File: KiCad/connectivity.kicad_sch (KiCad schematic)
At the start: 28 parts, among them IC17 GM02SP, U11 MAX98357A, U17 CXD5610GF, U18 ESP32-C6, U19 HP5354.A, U21 BGA524N6, U23 BGA524N6, Y1 WE-SPXO_CFPS-39, Y3 ECS-TXO-20CSMV4-260-AN-TR

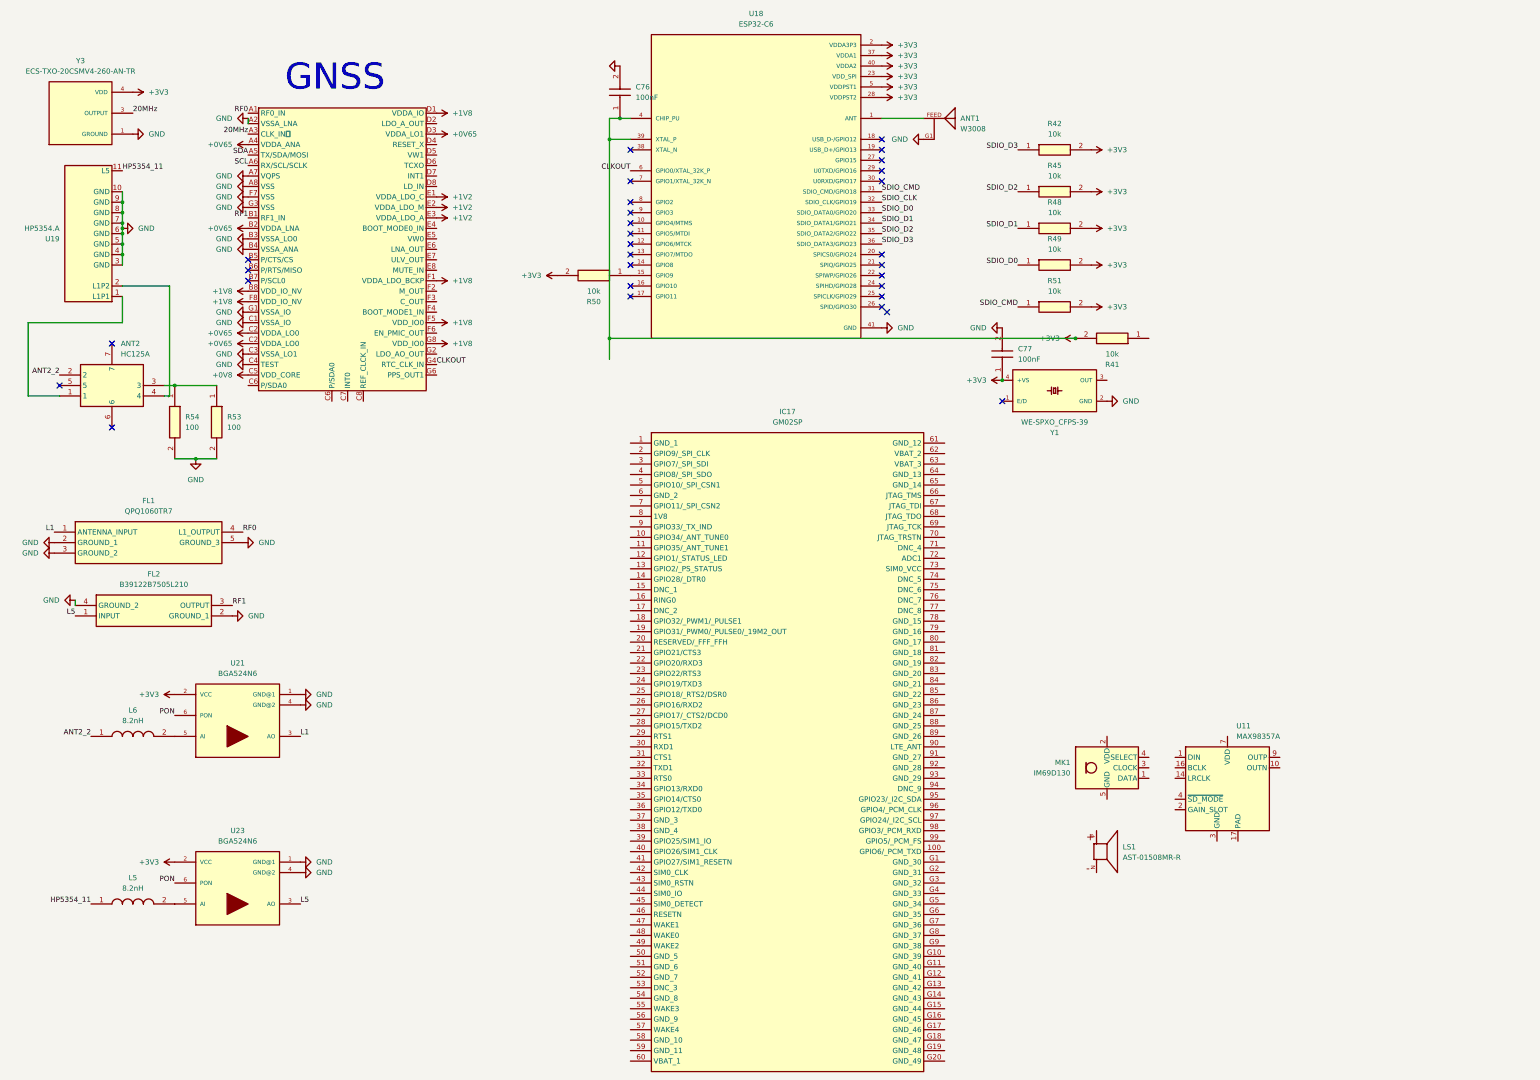
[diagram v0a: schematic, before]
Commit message: continue redesign
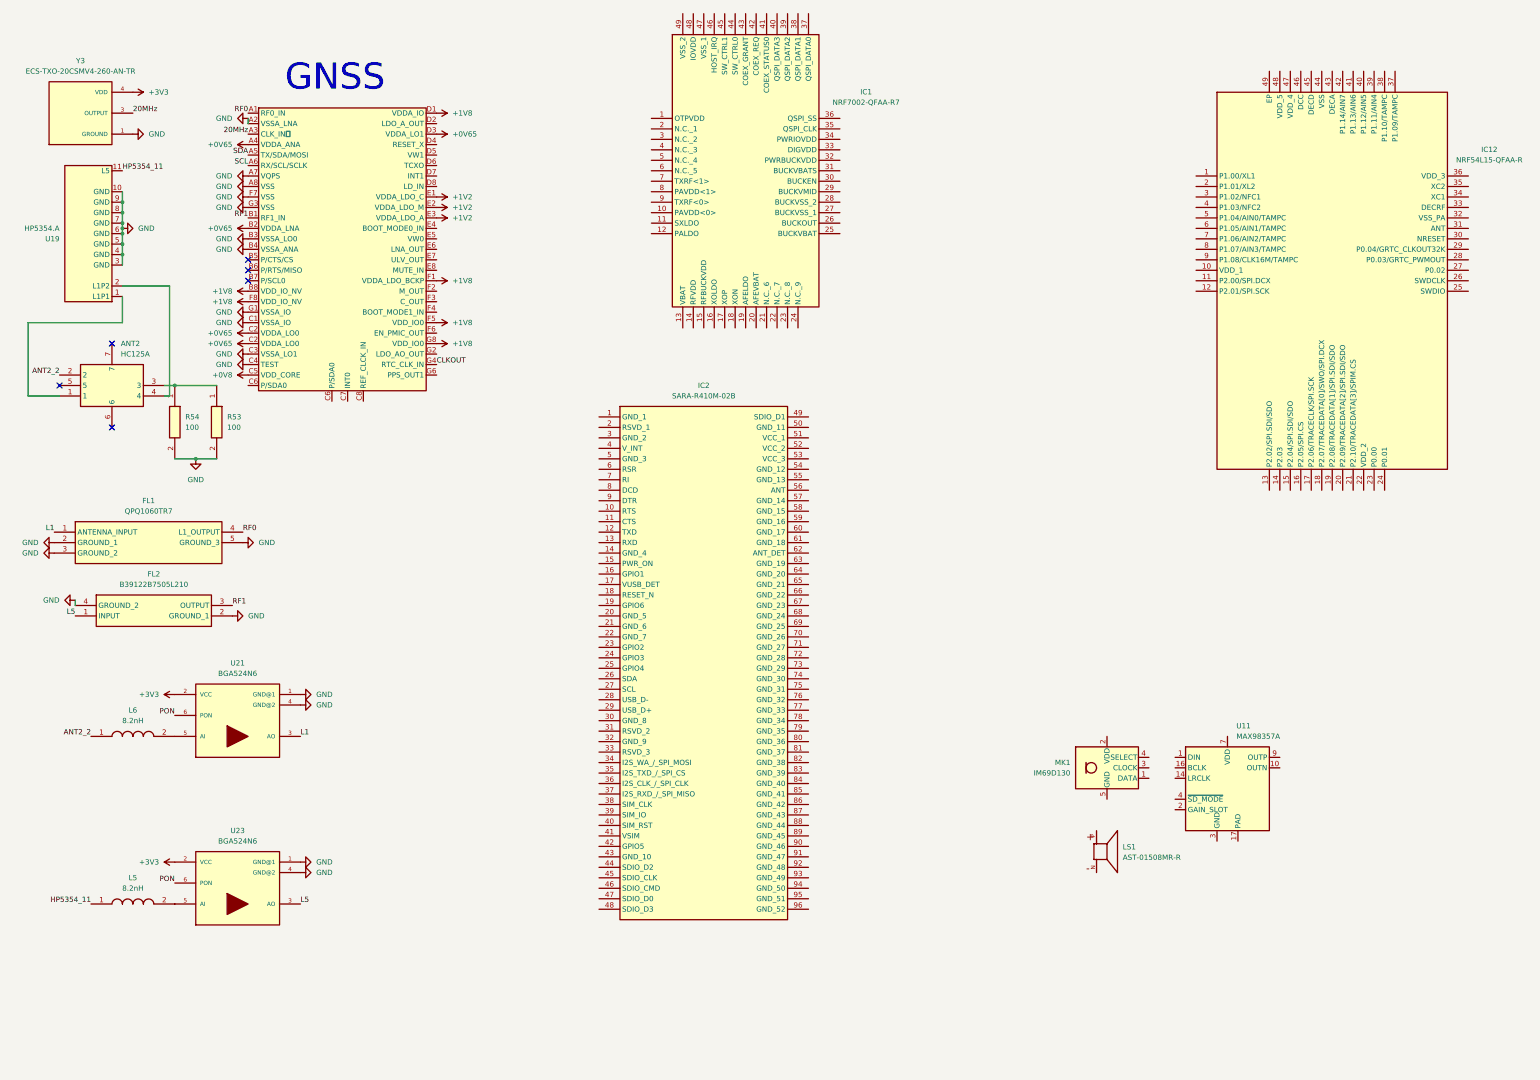
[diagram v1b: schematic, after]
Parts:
- removed ANT1: W3008, Footprints:ANTENNA_W3008, symbol Symbols:W3008
- removed C76, C77: 100nF, Footprints:GRM033D70J224ME01D, symbol Symbols:GRM033Z71C104KE14J
- removed IC17: GM02SP, Footprints:GM02SP, symbol Symbols:GM02SP
- removed R41, R42, R45, R48, R49, R50, R51: 10k, Footprints:ERJU01__0201_, symbol Symbols:ERJU01J103C
- removed U18: ESP32-C6, Footprints:ESP32-C6, symbol Symbols:ESP32-C6
- removed Y1: WE-SPXO_CFPS-39, Footprints:WE-SPXO_CFPS-39, symbol Symbols:WE-SPXO_CFPS-39
- added IC1: NRF7002-QFAA-R7, QFN40P600X600X95-49N, symbol Symbols:NRF7002-QFAA-R7
- added IC12: NRF54L15-QFAA-R, QFN40P600X600X95-49N, symbol Symbols:NRF54L15-QFAA-R
- added IC2: SARA-R410M-02B, SARAR412M02B, symbol Symbols:SARA-R410M-02B
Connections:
- no-connect marks 30 -> 6
